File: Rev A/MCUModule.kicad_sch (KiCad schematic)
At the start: 18 parts, among them U1 RaspberryPi_Pico, U2 74HC4051, U4 LM7805_TO220, U5 LM324

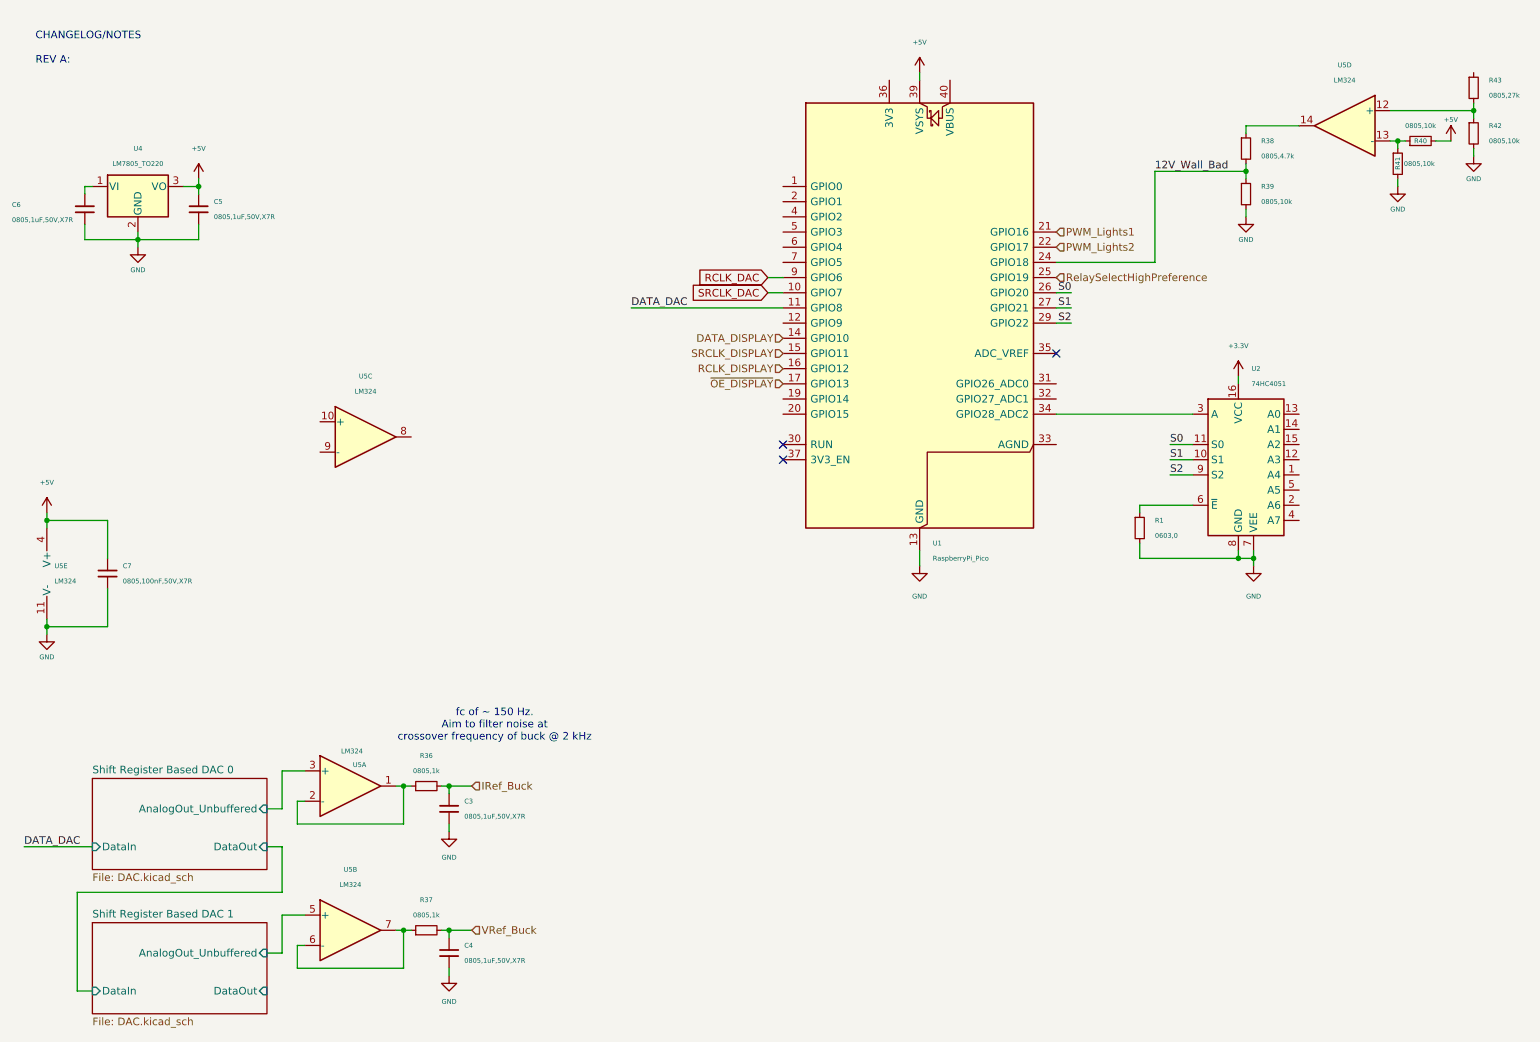
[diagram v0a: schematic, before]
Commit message: Update MCUModule.kicad_sch
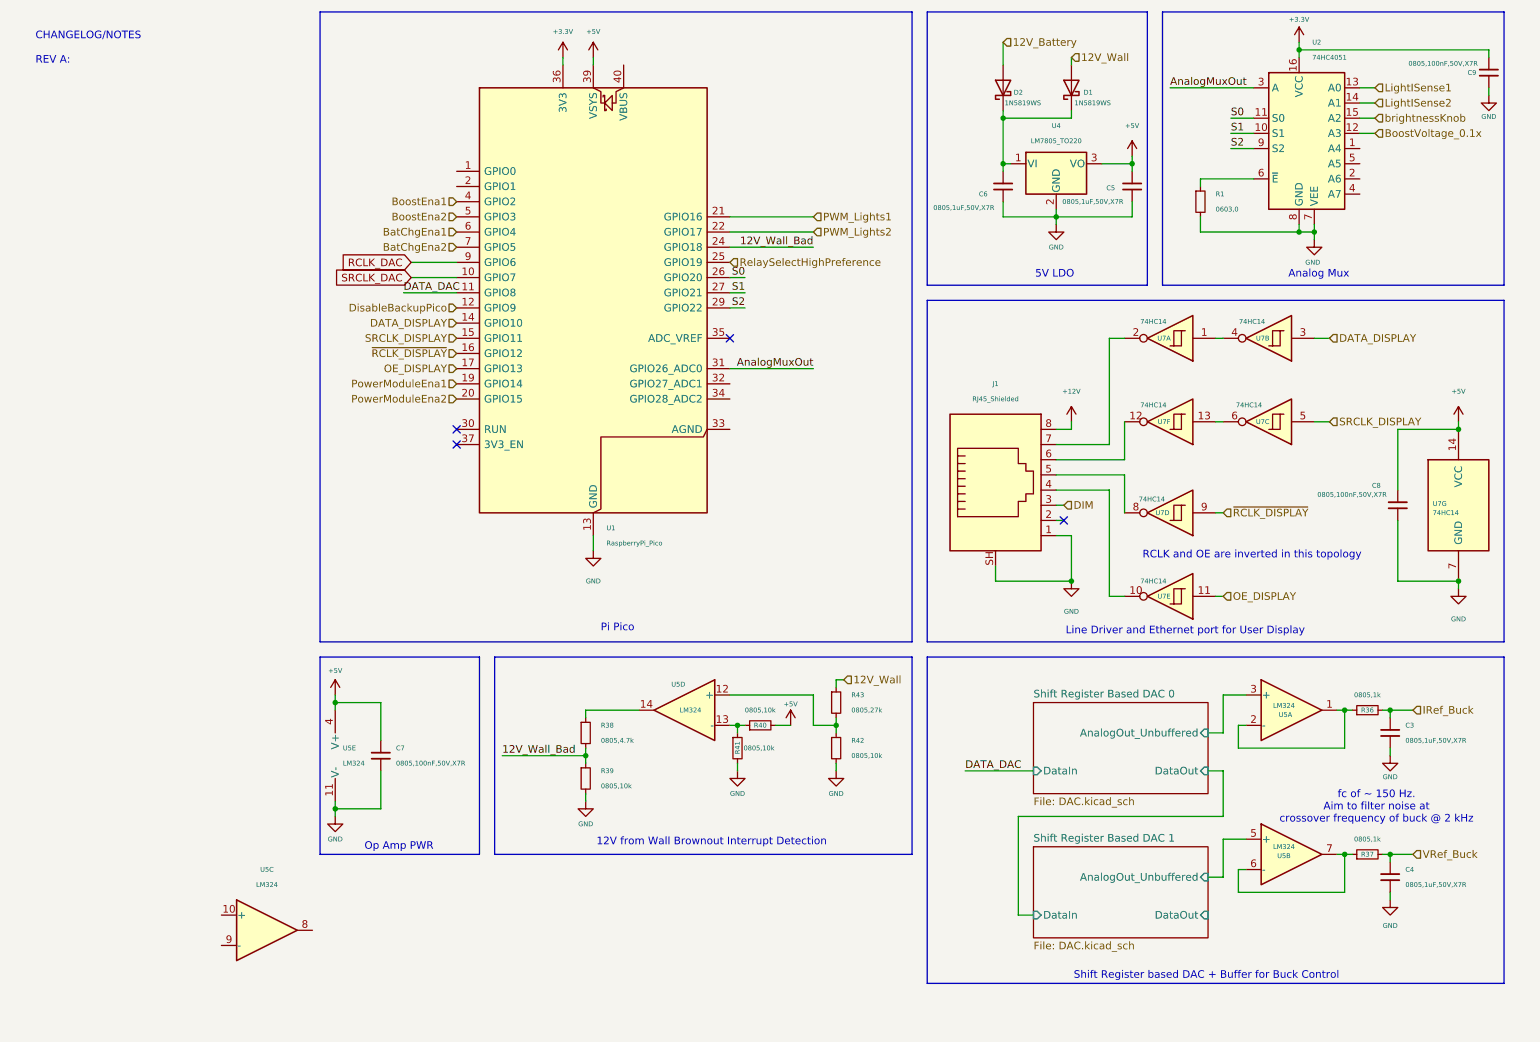
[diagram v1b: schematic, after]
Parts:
- added C8, C9: 0805,100nF,50V,X7R, C_0805_2012Metric, symbol jlcpcb-basic-capacitor:0805,100nF,50V,X7R
- added D1, D2: 1N5819WS, Diode_SMD:D_SOD-323, symbol Diode:1N5819WS
- added J1: RJ45_Shielded, Connector_RJ:RJ45_Shielded_EthernetJack, symbol Connector:RJ45_Shielded
- added U7: 74HC14, symbol 74xx:74HC14
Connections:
- net +3.3V: now also U1.36 (3V3), C9.1
- net +5V: now also C8.1, U7.14 (VCC)
- net DATA_DISPLAY: now also U7.3
- net GND: now also C8.2, C9.2, J1.1, J1.SH, U7.7 (GND)
- net SRCLK_DISPLAY: now also U7.5
- net at C6.1, U4.1 (VI): now also D1.1 (K), D2.1 (K)
- net 12V_Wall: now reaches R43.1
- net 12V_Wall: now also D1.2 (A)
- net BoostVoltage_0.1x: now reaches U2.12 (A3)
- net LightISense1: now reaches U2.13 (A0)
- net LightISense2: now reaches U2.14 (A1)
- net brightnessKnob: now reaches U2.15 (A2)
- net at U1.34 (GPIO28_ADC2): no longer U2.3 (A)
- net DisableBackupPico: now reaches U1.12 (GPIO9)
- net PowerModuleEna1: now reaches U1.19 (GPIO14)
- net PowerModuleEna2: now reaches U1.20 (GPIO15)
- net AnalogMuxOut: now reaches U1.31 (GPIO26_ADC0)
- net AnalogMuxOut: now also U2.3 (A)
- net BoostEna1: now reaches U1.4 (GPIO2)
- net BoostEna2: now reaches U1.5 (GPIO3)
- net BatChgEna1: now reaches U1.6 (GPIO4)
- net BatChgEna2: now reaches U1.7 (GPIO5)
- net RCLK_DISPLAY renamed ~{RCLK_DISPLAY}
- net ~{RCLK_DISPLAY}: now also U7.9
- net ~{OE_DISPLAY} renamed OE_DISPLAY
- net OE_DISPLAY: now also U7.11
- new net: U7.1, U7.4
- new net: J1.7, U7.2
- new net: J1.4, U7.10
- new net: J1.6, U7.12
- new net: U7.13, U7.6
- new net: J1.5, U7.8
- new net +12V: J1.8
- new net 12V_Battery: D2.2 (A)
- new net DIM: J1.3
- no-connect marks 3 -> 4
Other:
- note added: "12V from Wall Brownout Interrupt Detection"
- note added: "5V LDO"
- note added: "Analog Mux"
- note added: "Line Driver and Ethernet port for User Display"
- note added: "Op Amp PWR"
- note added: "Pi Pico"
- note added: "RCLK and OE are inverted in this topology"
- note added: "Shift Register based DAC + Buffer for Buck Control"
- moved on the sheet: C3, C4, C5, C6, C7, R1, R36, R37, R38, R39, R40, R41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
